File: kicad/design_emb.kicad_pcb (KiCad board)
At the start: 2 copper layers, 110 parts, among them J1 Conn_01x03, J2 Barrel_Jack, J3 USB_A, J4 Conn_01x03, J5 Conn_02x11_Counter_Clockwise, J6 Conn_02x10_Counter_Clockwise, J7 Screw_Terminal_01x02, J8 Screw_Terminal_01x02, K1 SANYOU_SRD_Form_C, K2 SANYOU_SRD_Form_C, Q1 MMBT3904, Q2 MMBT3904, U1 SRX.X.TCT, U10 S25FL116KOXNFIQ-11, U2 SRX.X.TCT, U3 STM32F446ZETx, U4 ICE40HX1K, U5 TLV1117LV33DCYR, U6 TLV1117LV33DCYR, U7 TLV1117LV12DCYR, U8 OMEGA2, U9 RCLAMP0502B

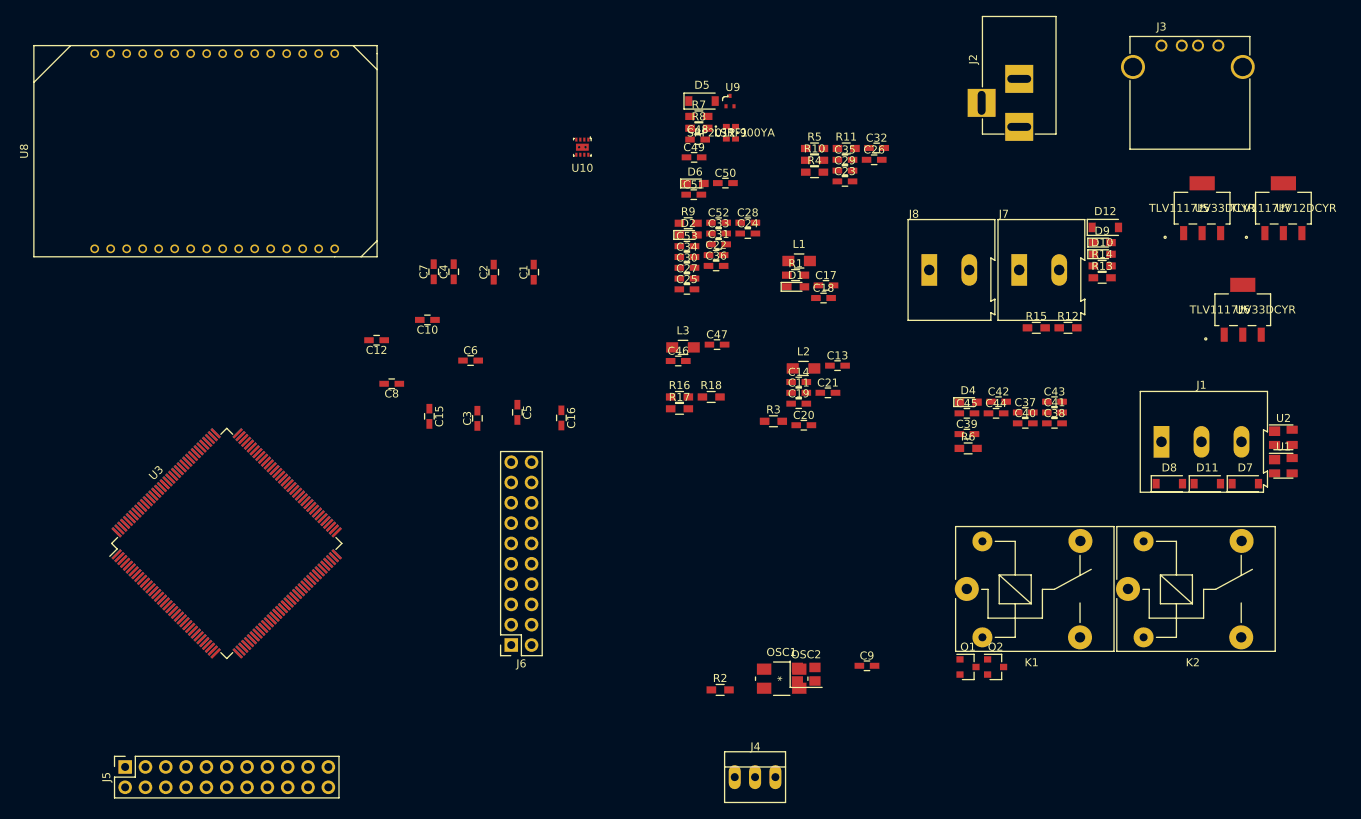
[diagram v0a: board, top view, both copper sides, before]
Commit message: design_emb.kicad_pcb
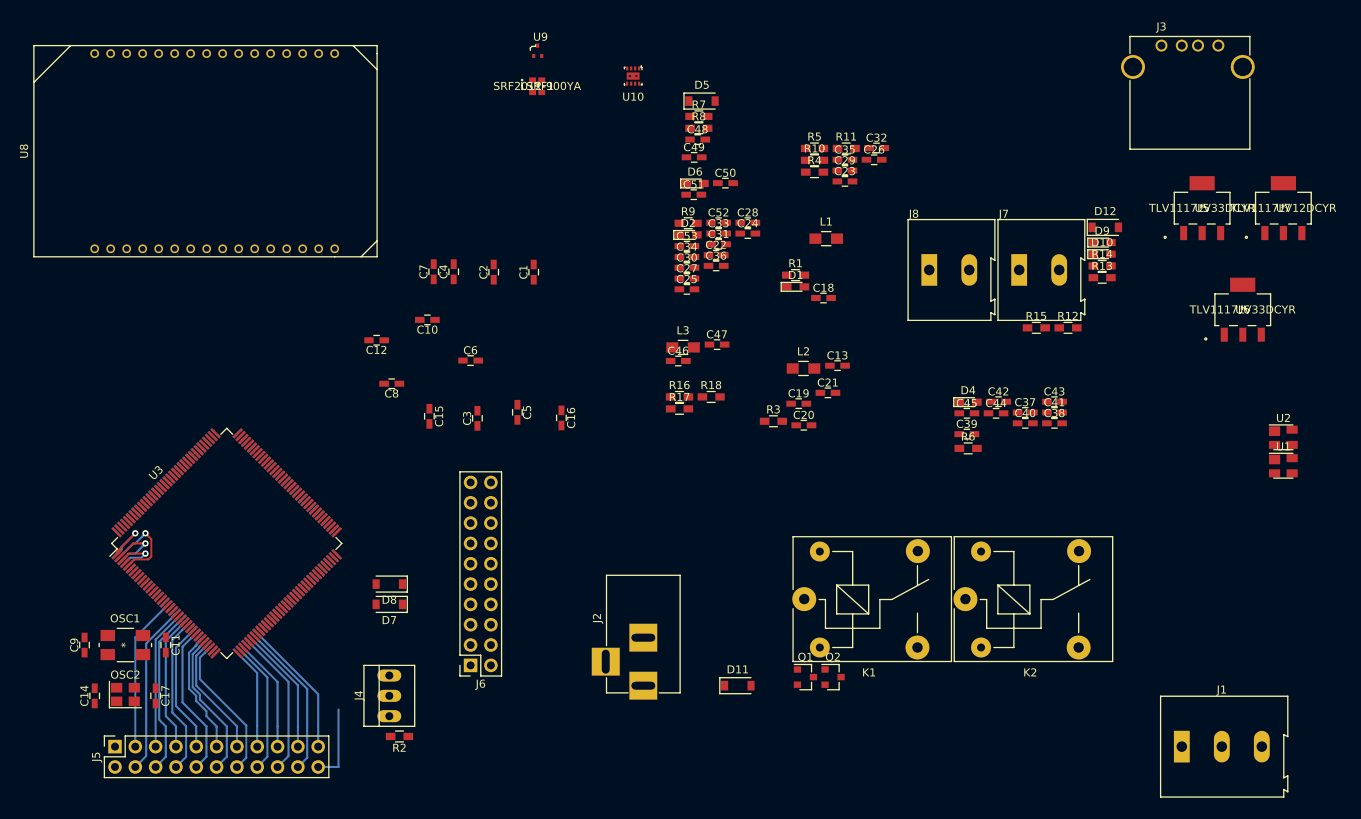
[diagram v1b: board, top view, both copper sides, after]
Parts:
- moved D7 108.1 mm to (72.4, 143.5), turned to 180 degrees
- moved D8 98.3 mm to (72.4, 141.0), turned to 180 degrees
- moved C17 98.3 mm to (43.2, 154.9), turned to 270 degrees
- moved C9 97.8 mm to (34.3, 148.6), turned to 90 degrees
- moved C14 96.4 mm to (35.6, 154.9), turned to 90 degrees
- moved C11 85.2 mm to (44.5, 148.6), turned to 270 degrees
- moved OSC2 85.1 mm to (39.4, 154.8)
- moved J2 84.2 mm to (104.1, 153.7)
- moved OSC1 82.2 mm to (39.4, 148.6)
- moved D11 63.9 mm to (116.0, 153.7)
- moved J4 43.8 mm to (72.4, 157.5), turned to 90 degrees
- moved R2 40.5 mm to (73.7, 160.0), turned to 180 degrees
- moved J1 38.2 mm to (171.4, 161.3)
- moved LSRF1 24.9 mm to (90.9, 78.7)
- moved U9 24.8 mm to (90.9, 74.3)
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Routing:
- net /sheet3/GPIO1: track 0.00 -> 21.3 mm
- net /sheet3/GPIO3: track 0.00 -> 20.5 mm
- net /sheet3/GPIO5: track 0.00 -> 19.8 mm
- net /sheet3/GPIO17: track 0.00 -> 19.5 mm
- net /sheet3/GPIO0: track 0.00 -> 19.3 mm
- net /sheet3/GPIO7: track 0.00 -> 19.1 mm
- net /sheet3/GPIO9: track 0.00 -> 18.5 mm
- net /sheet3/GPIO11: track 0.00 -> 18.3 mm
- net /sheet3/GPIO15: track 0.00 -> 18.2 mm
- net /sheet3/GPIO2: track 0.00 -> 17.5 mm
- net /sheet3/GPIO18: track 0.00 -> 17.3 mm
- net /sheet3/GPIO4: track 0.00 -> 17.0 mm
- net /sheet3/GPIO13: track 0.00 -> 16.5 mm
- net /sheet3/GPIO6: track 0.00 -> 16.4 mm
- net /sheet3/GPIO16: track 0.00 -> 15.8 mm
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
